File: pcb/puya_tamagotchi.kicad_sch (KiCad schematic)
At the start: 31 parts, among them J1 FLASHING ONLY, J2 ADDITIONAL, Q1 2N7002, SW1 TS-1187A-B-A-B, SW2 TS-1187A-B-A-B, SW3 TS-1187A-B-A-B, SW4 TS-1187A-B-A-B, U1 PY32F002BF15U6TR, U2 OLED_128x64_SSD1306

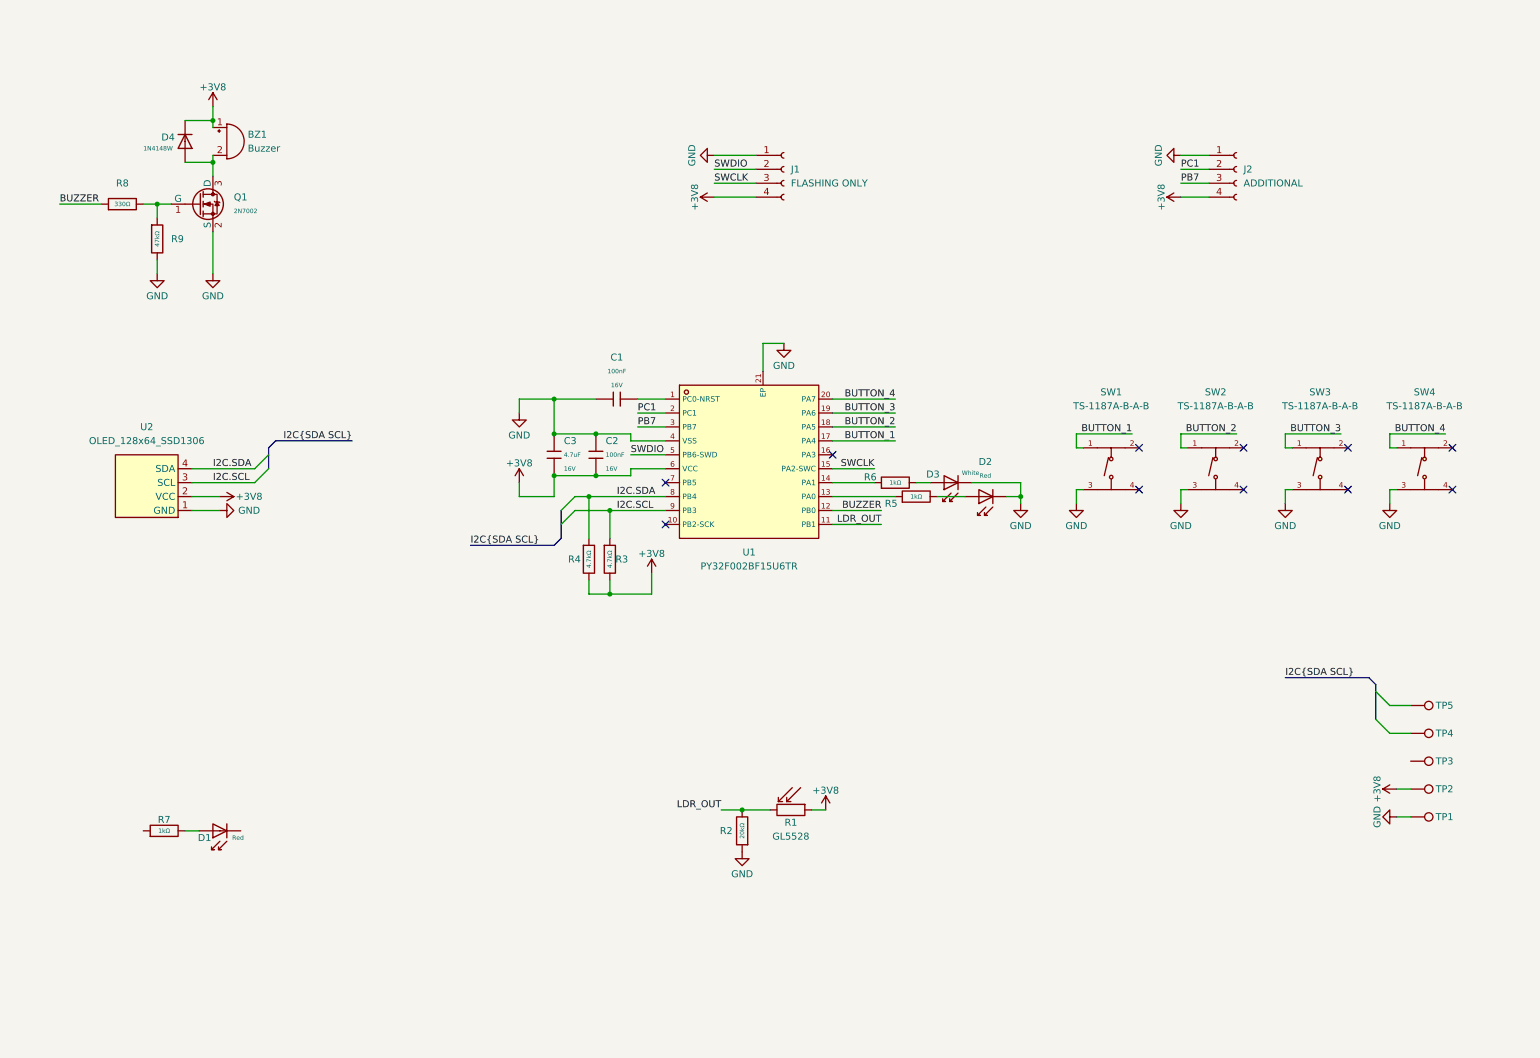
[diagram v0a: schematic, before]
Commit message: Add charging and protection, clean schematic
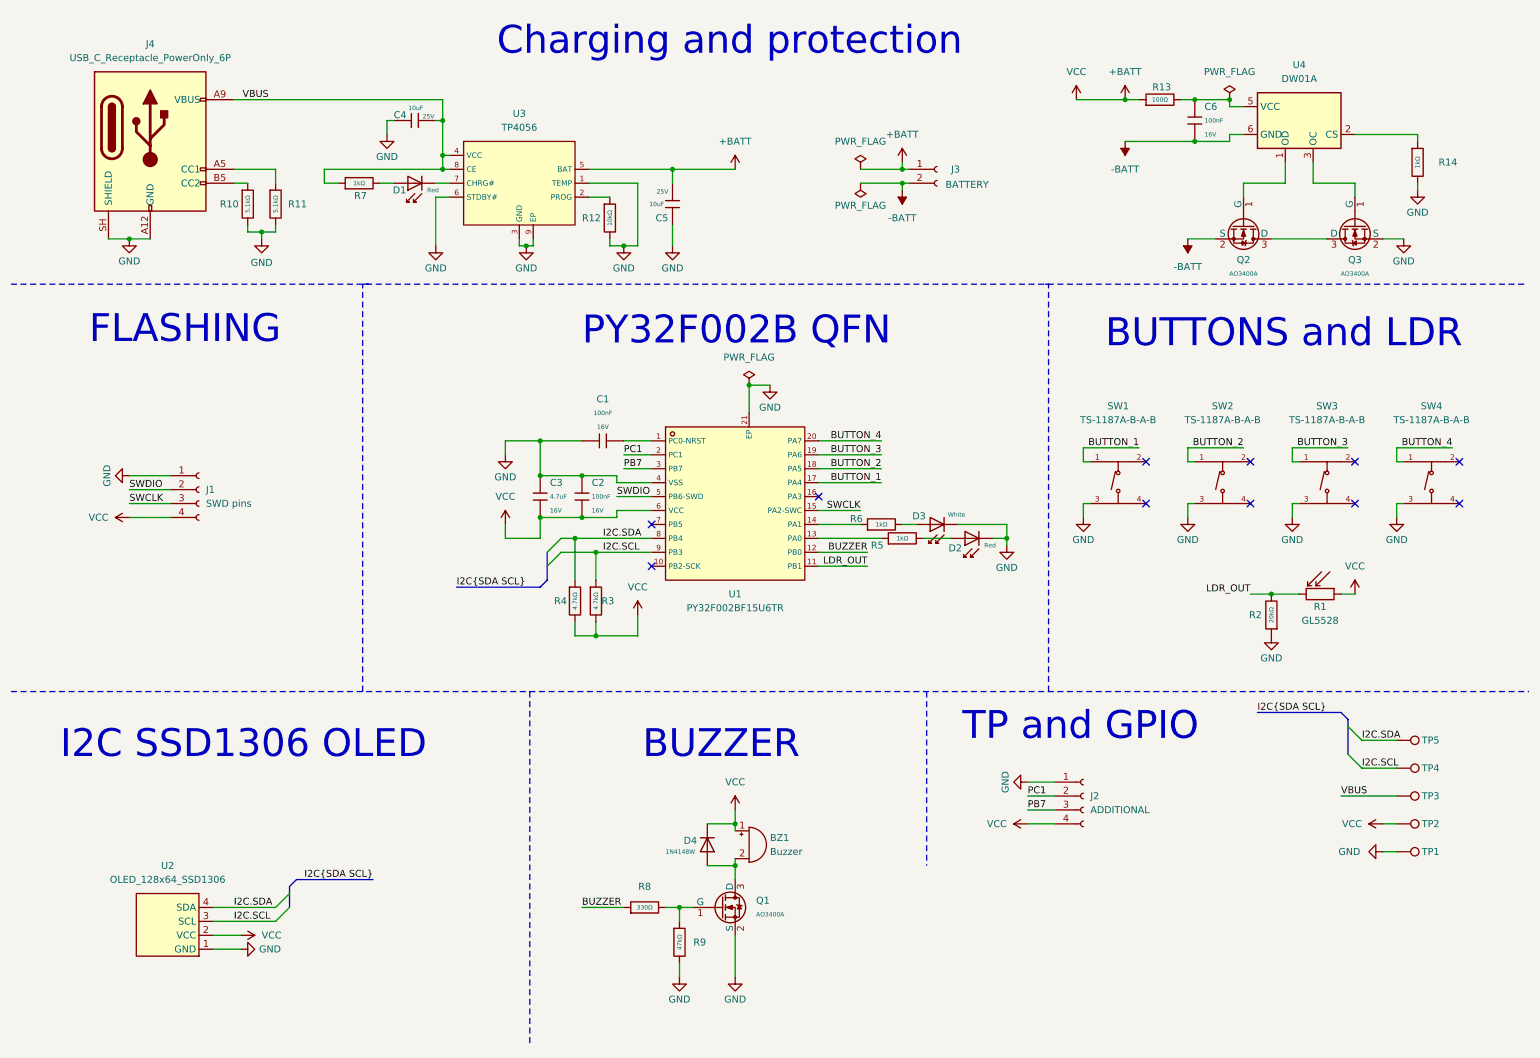
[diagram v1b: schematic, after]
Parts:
- removed Q1: 2N7002, PCM_JLCPCB:Q_SOT-23, symbol PCM_JLCPCB-Transistors:NMOS,2N7002
- added C4, C5: 10uF, PCM_JLCPCB:C_0603, symbol PCM_JLCPCB-Capacitors:0603,10uF,(2)
- added C6: 100nF, PCM_JLCPCB:C_0402, symbol PCM_JLCPCB-Capacitors:0402,100nF
- added J3: BATTERY, Connector_JST:JST_EH_B2B-EH-A_1x02_P2.50mm_Vertical, symbol Connector:Conn_01x02_Socket
- added J4: USB_C_Receptacle_PowerOnly_6P, Connector_USB:USB_C_Receptacle_HRO_TYPE-C-31-M-17, symbol Connector:USB_C_Receptacle_PowerOnly_6P
- added Q1, Q2, Q3: AO3400A, PCM_JLCPCB:Q_SOT-23, symbol PCM_JLCPCB-Transistors:NMOS,AO3400A
- added R10, R11: 5.1kΩ, PCM_JLCPCB:R_0402, symbol PCM_JLCPCB-Resistors:0402,5.1kΩ
- added R12: 10kΩ, PCM_JLCPCB:R_0402, symbol PCM_JLCPCB-Resistors:0402,10kΩ
- added R13: 100Ω, PCM_JLCPCB:R_0402, symbol PCM_JLCPCB-Resistors:0402,100Ω
- added R14: 1kΩ, PCM_JLCPCB:R_0402, symbol PCM_JLCPCB-Resistors:0402,1kΩ
- added U3: TP4056, PCM_JLCPCB:ESOP-8_L4.9-W3.9-P1.27-LS6.0-BL-EP, symbol PCM_JLCPCB-Power:Battery, Li-Ion, 1.0A, TP4056
- added U4: DW01A, Package_TO_SOT_SMD:SOT-23-6, symbol Battery_Management:DW01A
- J1: value FLASHING ONLY -> SWD pins
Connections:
- net GND: now also C4.1, C5.1, J4.A12 (GND), J4.B12 (GND), J4.SH (SHIELD), Q1.2 (S), Q3.2 (S), R10.2, R11.2, R12.2, R14.2, U3.1 (TEMP), U3.3 (GND), U3.6 (STDBY#), U3.9 (EP)
- net I2C.SCL: now also TP4.1
- net I2C.SDA: now also TP5.1
- net at R8.2, R9.1: now also Q1.1 (G)
- net VBUS: now reaches R7.1
- net VBUS: now also TP3.1, C4.2, J4.A9 (VBUS), J4.B9 (VBUS), U3.4 (VCC), U3.8 (CE)
- net at BZ1.2 (-), D4.2: now also Q1.3 (D)
- net at D1.1: now also U3.7 (CHRG#)
- net +3V8 renamed +BATT
- net +BATT: now also C5.2, J3.1 (Pin_1), R13.1, U3.5 (BAT)
- new net: J4.B5 (CC2), R10.1
- new net: C6.1, R13.2, U4.5 (VCC)
- new net: Q2.1 (G), U4.1 (OD)
- new net: Q2.3 (D), Q3.3 (D)
- new net: Q3.1 (G), U4.3 (OC)
- new net: J4.A5 (CC1), R11.1
- new net: R12.1, U3.2 (PROG)
- new net: R14.1, U4.2 (CS)
- new net -BATT: C6.2, J3.2 (Pin_2), Q2.2 (S), U4.6 (GND)
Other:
- note added: "BUTTONS and LDR"
- note added: "BUZZER"
- note added: "Charging and protection"
- note added: "FLASHING"
- note added: "I2C SSD1306 OLED"
- note added: "PY32F002B QFN"
- note added: "TP and GPIO"
- moved on the sheet: BZ1, C1, C2, C3, D1, D2, D3, D4, J1, J2, R1, R2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
